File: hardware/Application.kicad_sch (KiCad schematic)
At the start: 33 parts, among them J501 Conn_ARM_SWD_TagConnect_TC203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, J502 Conn_ARM_SWD_TagConnect_TC2030, J503 BOOT0, J504 USB_B, U501 STM32G431CBU6, U502 W25X10CLUXIG, Y501 32_Mhz

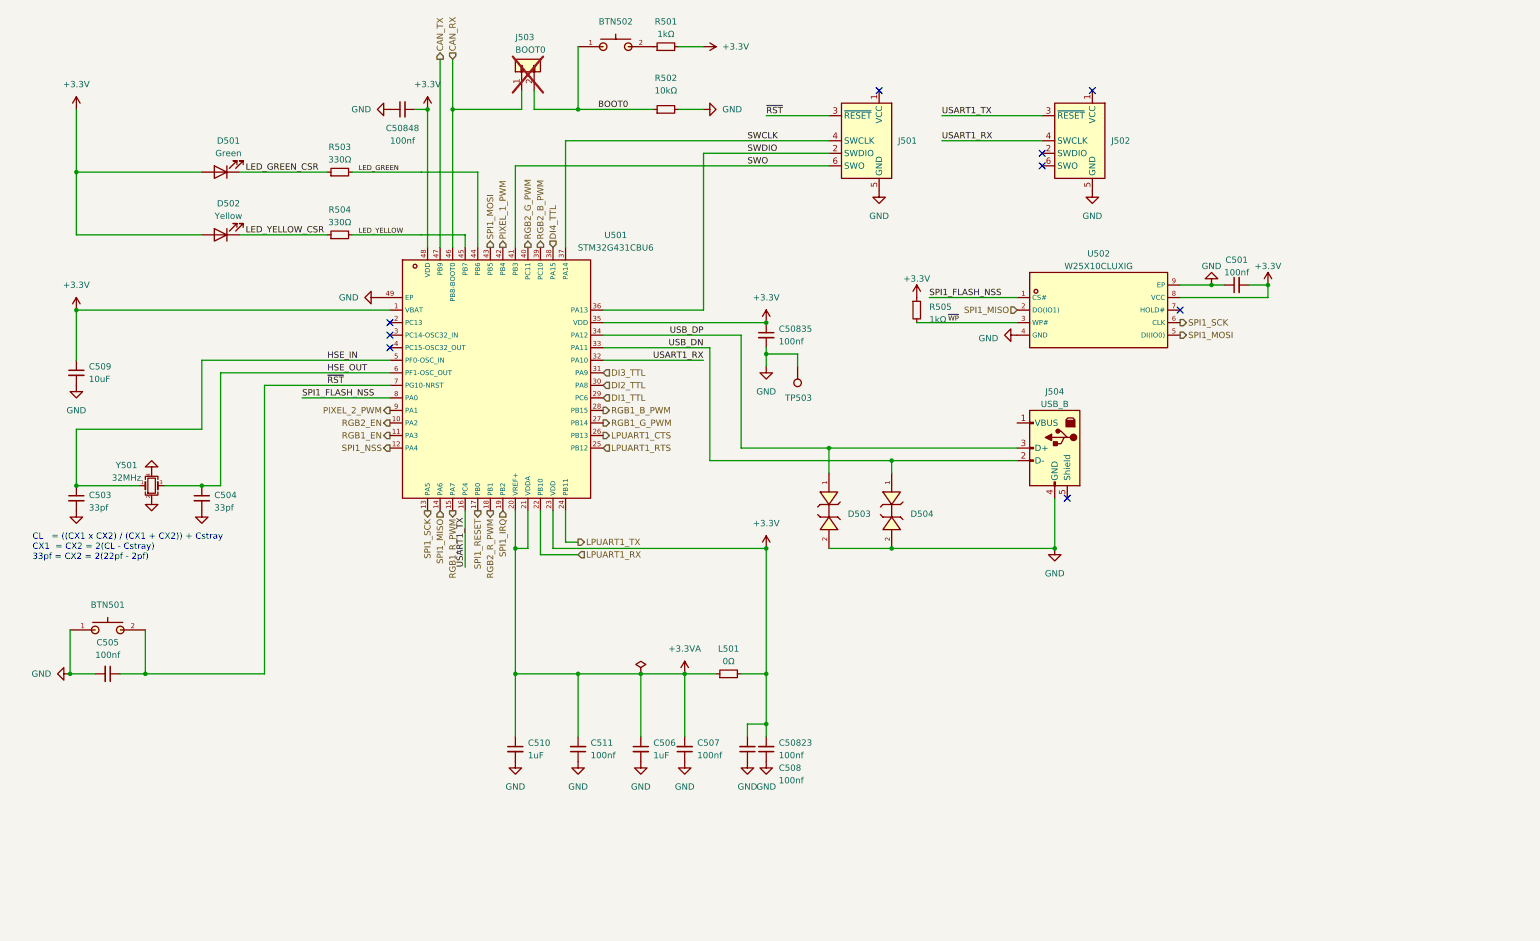
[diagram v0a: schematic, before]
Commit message: Rev 2 submitted for production
Signed-off-by: Connor Rigby <connorr@hey.com>
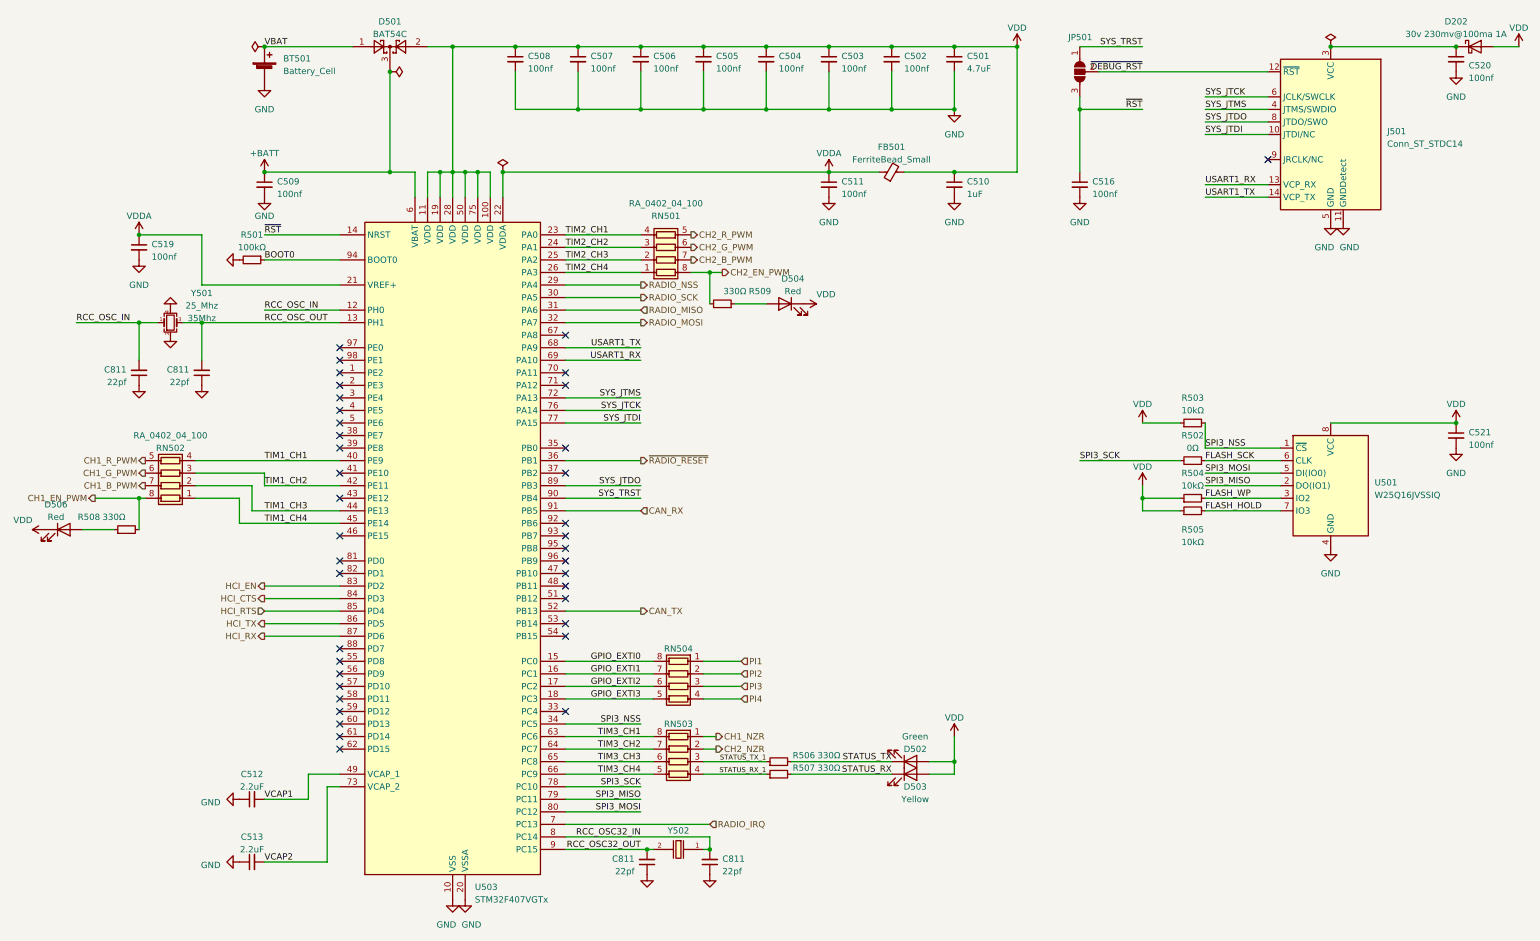
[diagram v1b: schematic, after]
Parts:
- removed BTN501, BTN502: GT-TC029B-H025-L1N, Button:SW-SMD_L3.9-W3.0-P4.45, symbol LCSC_Tactile_Switch:GT-TC029B-H025-L1N
- removed C501, C50823, C50835, C50848: C_0402_100nf_X7R, Capacitor_SMD:C_0402_1005Metric, symbol LCSC_Capacitor:C_0402_100nf_X7R
- removed C503, C504: C_0402_33p_C0G, Capacitor_SMD:C_0402_1005Metric, symbol LCSC_Capacitor:C_0402_33p_C0G
- removed C506: C_0402_1u_X5R, Capacitor_SMD:C_0402_1005Metric, symbol LCSC_Capacitor:C_0402_1u_X5R
- removed C509: C_0805_10u_X5R, Capacitor_SMD:C_0805_2012Metric, symbol LCSC_Capacitor:C_0805_10u_X5R
- removed D501: LED_0603_GREEN, LED_SMD:LED_0603_1608Metric, symbol LCSC_LED:LED_0603_GREEN
- removed D502: LED_0603_YELLOW, LED_SMD:LED_0603_1608Metric, symbol LCSC_LED:LED_0603_YELLOW
- removed D503, D504: ESD9B3_3ST5G, LCSC_ESD:SOD-923_L0.8-W0.6-LS1.0-BI-1, symbol LCSC_ESD:ESD9B3_3ST5G
- removed J501: Conn_ARM_SWD_TagConnect_TC2030-NL, Connector:Tag-Connect_TC2030-IDC-NL_2x03_P1.27mm_Vertical, symbol Connector:Conn_ARM_SWD_TagConnect_TC2030-NL
- removed J502: Conn_ARM_SWD_TagConnect_TC2030, Connector:Tag-Connect_TC2030-IDC-FP_2x03_P1.27mm_Vertical, symbol Connector:Conn_ARM_SWD_TagConnect_TC2030
- removed J503: BOOT0, Connector_PinHeader_2.54mm:PinHeader_1x02_P2.54mm_Vertical, symbol Connector_Generic:Conn_01x02
- removed J504: USB_B, LCSC_Connector:USB-B-TH_67068-8000, symbol Connector:USB_B
- removed L501: R_0402_0, Resistor_SMD:R_0402_1005Metric, symbol LCSC_Resistor:R_0402_0
- removed R501, R505: R_0402_1k, Resistor_SMD:R_0402_1005Metric, symbol LCSC_Resistor:R_0402_1k
- removed R502: R_0402_10k, Resistor_SMD:R_0402_1005Metric, symbol LCSC_Resistor:R_0402_10k
- removed R503, R504: R_0603_330, Resistor_SMD:R_0603_1608Metric, symbol LCSC_Resistor:R_0603_330
- removed TP503: GND, TestPoint:TestPoint_Pad_D1.0mm, symbol Connector:TestPoint
- removed U501: STM32G431CBU6, LCSC_Microcontroller:QFN50P700X700X60-49N, symbol LCSC_Microcontroller:STM32G431CBU6
- removed U502: W25X10CLUXIG, LCSC_Microcontroller:USON-8_L3.0-W2.0-P0.50-BL-EP-1, symbol LCSC_Microcontroller:W25X10CLUXIG
- removed Y501: 32_Mhz, Crystal:Crystal_SMD_3225-4Pin_3.2x2.5mm, symbol LCSC_Crystal:32_Mhz
- added BT501: Battery_Cell, LCSC_Connector:BAT-SMD_CR1220-2, symbol Device:Battery_Cell
- added C501: C_0805_4u7_X5R, Capacitor_SMD:C_0805_2012Metric, symbol LCSC_Capacitor:C_0805_4u7_X5R
- added C502, C503, C504, C506, C509, C516, C519, C520, C521: C_0402_100nf_X7R, Capacitor_SMD:C_0402_1005Metric, symbol LCSC_Capacitor:C_0402_100nf_X7R
- added C512, C513: C_0402_2u2_X5R, Capacitor_SMD:C_0402_1005Metric, symbol LCSC_Capacitor:C_0402_2u2_X5R
- added C811 (x4): C_0402_22p_C0G, Capacitor_SMD:C_0402_1005Metric, symbol LCSC_Capacitor:C_0402_22p_C0G
- added D202: 30v 230mv@100ma 1A, Diode_SMD:D_SOD-323F, symbol Device:D_Schottky
- added D501: BAT54C, Package_TO_SOT_SMD:SOT-23, symbol Diode:BAT54C
- added D502: LED_0603_GREEN, LED_SMD:LED_0603_1608Metric, symbol LCSC_LED:LED_0603_GREEN
- added D503: LED_0603_YELLOW, LED_SMD:LED_0603_1608Metric, symbol LCSC_LED:LED_0603_YELLOW
- added D504, D506: LED_0603_RED, LED_SMD:LED_0603_1608Metric, symbol LCSC_LED:LED_0603_RED
- added FB501: FerriteBead_Small, Inductor_SMD:L_0402_1005Metric, symbol Device:FerriteBead_Small
- added J501: Conn_ST_STDC14, LCSC_Connector:TC2070-IDC-FP, symbol Connector:Conn_ST_STDC14
- added JP501: SolderJumper_3_Open, Jumper:SolderJumper-3_P1.3mm_Open_RoundedPad1.0x1.5mm_NumberLabels, symbol Jumper:SolderJumper_3_Open
- added R501: R_0402_100k, Resistor_SMD:R_0402_1005Metric, symbol LCSC_Resistor:R_0402_100k
- added R502: R_0402_0, Resistor_SMD:R_0402_1005Metric, symbol LCSC_Resistor:R_0402_0
- added R503, R504, R505: R_0402_10k, Resistor_SMD:R_0402_1005Metric, symbol LCSC_Resistor:R_0402_10k
- added R506, R507, R508, R509: R_0603_330, Resistor_SMD:R_0603_1608Metric, symbol LCSC_Resistor:R_0603_330
- added RN501, RN502, RN503, RN504: RA_0402_04_100, Resistor_SMD:R_Array_Concave_4x0402, symbol LCSC_Resistor:RA_0402_04_100
- added U501: W25Q16JVSSIQ, Package_SO:SOIC-8_5.23x5.23mm_P1.27mm, symbol LCSC_Microcontroller:W25Q16JVSSIQ
- added U503: STM32F407VGTx, Package_QFP:LQFP-100_14x14mm_P0.5mm, symbol MCU_ST_STM32F4:STM32F407VGTx
- added Y501: 25_Mhz, Crystal:Crystal_SMD_3225-4Pin_3.2x2.5mm, symbol LCSC_Crystal:25_Mhz
- added Y502: Q13FC1350000400, Crystal:Crystal_SMD_3215-2Pin_3.2x1.5mm, symbol LCSC_Crystal:Q13FC1350000400
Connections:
- net +3.3V is gone; now on net GND: C508.2
- net BOOT0: now also R501.1, U503.94 (BOOT0)
- net CAN_RX: now also U503.91 (PB5)
- net CAN_TX: now also U503.52 (PB13)
- net GND: now also C507.2, C511.2, BT501.2 (-), C501.2, C502.2, C503.2, C504.2, C506.2, C509.2, C512.1, C513.1, C516.2, C519.2, C520.2, C521.2, C811.1, C811.1, C811.1, C811.1, J501.11 (GNDDetect), J501.5 (GND), J501.7 (GND), R501.2, U501.4 (GND), U503.10 (VSS), U503.20 (VSSA), U503.27 (VSS), U503.74 (VSS), U503.99 (VSS), Y501.2, Y501.4; no longer C507.1, C508.1, C511.1
- net USART1_RX: now also J501.13 (VCP_RX), U503.69 (PA10)
- net USART1_TX: now also J501.14 (VCP_TX), U503.68 (PA9)
- net ~{RST}: now also C516.1, JP501.3 (B), U503.14 (NRST); no longer C505.1
- removed net +3.3VA: C507.2, C510.1, C511.2
- new net: D504.2 (A), R509.1
- new net: C520.1, D202.1 (K), J501.3 (VCC)
- new net: D506.2 (A), R508.1
- new net +BATT: C509.1, D501.3, U503.6 (VBAT)
- new net CH1_B_PWM: RN502.7 (R2.2)
- new net CH1_EN_PWM: R508.2, RN502.8 (R1.2)
- new net CH1_G_PWM: RN502.6 (R3.2)
- new net CH1_NZR: RN503.1 (R1.1)
- new net CH1_R_PWM: RN502.5 (R4.2)
- new net CH2_B_PWM: RN501.7 (R2.2)
- new net CH2_EN_PWM: R509.2, RN501.8 (R1.2)
- new net CH2_G_PWM: RN501.6 (R3.2)
- new net CH2_NZR: RN503.2 (R2.1)
- new net CH2_R_PWM: RN501.5 (R4.2)
- new net FLASH_HOLD: R505.2, U501.7 (IO3)
- new net FLASH_SCK: R502.1, U501.6 (CLK)
- new net FLASH_WP: R504.2, U501.3 (IO2)
- new net GPIO_EXTI0: RN504.8 (R1.2), U503.15 (PC0)
- new net GPIO_EXTI1: RN504.7 (R2.2), U503.16 (PC1)
- new net GPIO_EXTI2: RN504.6 (R3.2), U503.17 (PC2)
- new net GPIO_EXTI3: RN504.5 (R4.2), U503.18 (PC3)
- new net HCI_CTS: U503.84 (PD3)
- new net HCI_EN: U503.83 (PD2)
- new net HCI_RTS: U503.85 (PD4)
- new net HCI_RX: U503.87 (PD6)
- new net HCI_TX: U503.86 (PD5)
- new net PI1: RN504.1 (R1.1)
- new net PI2: RN504.2 (R2.1)
- new net PI3: RN504.3 (R3.1)
- new net PI4: RN504.4 (R4.1)
- new net RADIO_IRQ: U503.7 (PC13)
- new net RADIO_MISO: U503.31 (PA6)
- new net RADIO_MOSI: U503.32 (PA7)
- new net RADIO_NSS: U503.29 (PA4)
- new net RADIO_SCK: U503.30 (PA5)
- new net RCC_OSC32_IN: C811.2, U503.8 (PC14), Y502.1
- new net RCC_OSC32_OUT: C811.2, U503.9 (PC15), Y502.2
- new net RCC_OSC_IN: C811.2, U503.12 (PH0), Y501.1
- new net RCC_OSC_OUT: C811.2, U503.13 (PH1), Y501.3
- new net SPI3_MISO: U501.2 (DO(IO1)), U503.79 (PC11)
- new net SPI3_MOSI: U501.5 (DI(IO0)), U503.80 (PC12)
- new net SPI3_NSS: R503.2, U501.1 (~{CS}), U503.34 (PC5)
- new net SPI3_SCK: R502.2, U503.78 (PC10)
- new net STATUS_RX: D503.1 (K), R507.2
- new net STATUS_RX_1: R507.1, RN503.4 (R4.1)
- new net STATUS_TX: D502.1 (K), R506.2
- new net STATUS_TX_1: R506.1, RN503.3 (R3.1)
- new net SYS_JTCK: J501.6 (JCLK/SWCLK), U503.76 (PA14)
- new net SYS_JTDI: J501.10 (JTDI/NC), U503.77 (PA15)
- new net SYS_JTDO: J501.8 (JTDO/SWO), U503.89 (PB3)
- new net SYS_JTMS: J501.4 (JTMS/SWDIO), U503.72 (PA13)
- new net SYS_TRST: JP501.1 (A), U503.90 (PB4)
- new net TIM1_CH1: RN502.4 (R4.1), U503.40 (PE9)
- new net TIM1_CH2: RN502.3 (R3.1), U503.42 (PE11)
- new net TIM1_CH3: RN502.2 (R2.1), U503.44 (PE13)
- new net TIM1_CH4: RN502.1 (R1.1), U503.45 (PE14)
- new net TIM2_CH1: RN501.4 (R4.1), U503.23 (PA0)
- new net TIM2_CH2: RN501.3 (R3.1), U503.24 (PA1)
- new net TIM2_CH3: RN501.2 (R2.1), U503.25 (PA2)
- new net TIM2_CH4: RN501.1 (R1.1), U503.26 (PA3)
- new net TIM3_CH1: RN503.8 (R1.2), U503.63 (PC6)
- new net TIM3_CH2: RN503.7 (R2.2), U503.64 (PC7)
- new net TIM3_CH3: RN503.6 (R3.2), U503.65 (PC8)
- new net TIM3_CH4: RN503.5 (R4.2), U503.66 (PC9)
- new net VBAT: BT501.1 (+), D501.1
- new net VCAP1: C512.2, U503.49 (VCAP_1)
- new net VCAP2: C513.2, U503.73 (VCAP_2)
- new net VDD: C501.1, C502.1, C503.1, C504.1, C505.1, C506.1, C507.1, C508.1, C510.1, C521.1, D202.2 (A), D501.2, D502.2 (A), D503.2 (A), D504.1 (K), D506.1 (K), FB501.2, R503.1, R504.1, R505.1, U501.8 (VCC), U503.100 (VDD), U503.11 (VDD), U503.19 (VDD), U503.28 (VDD), U503.50 (VDD), U503.75 (VDD)
- new net VDDA: C511.1, C519.1, FB501.1, U503.21 (VREF+), U503.22 (VDDA)
- new net ~{DEBUG_RST}: J501.12 (~{RST}), JP501.2 (C)
- new net ~{RADIO_RESET}: U503.36 (PB1)
- no-connect marks 9 -> 39
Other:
- note removed: "CL = ((CX1 x CX2) / (CX1 + CX2)) + Cstray CX1 = CX2 = 2(CL - Cstray) 33pf = CX2 = 2(22pf - 2pf)"
